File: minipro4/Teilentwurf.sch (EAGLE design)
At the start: 90 parts, among them IC1 MEGA8-P, IC2 FT232RL_ADAPTER, IC3 78L08Z, IC4 4051N, IC5 TL082P, IC6 4051N, IC7 TL082P, J1 HOHLSTECKER, Q2 BS170, Q3 BS170, Q4 BS170, Q6 IRF4905, X1 , X2 CON_COAX

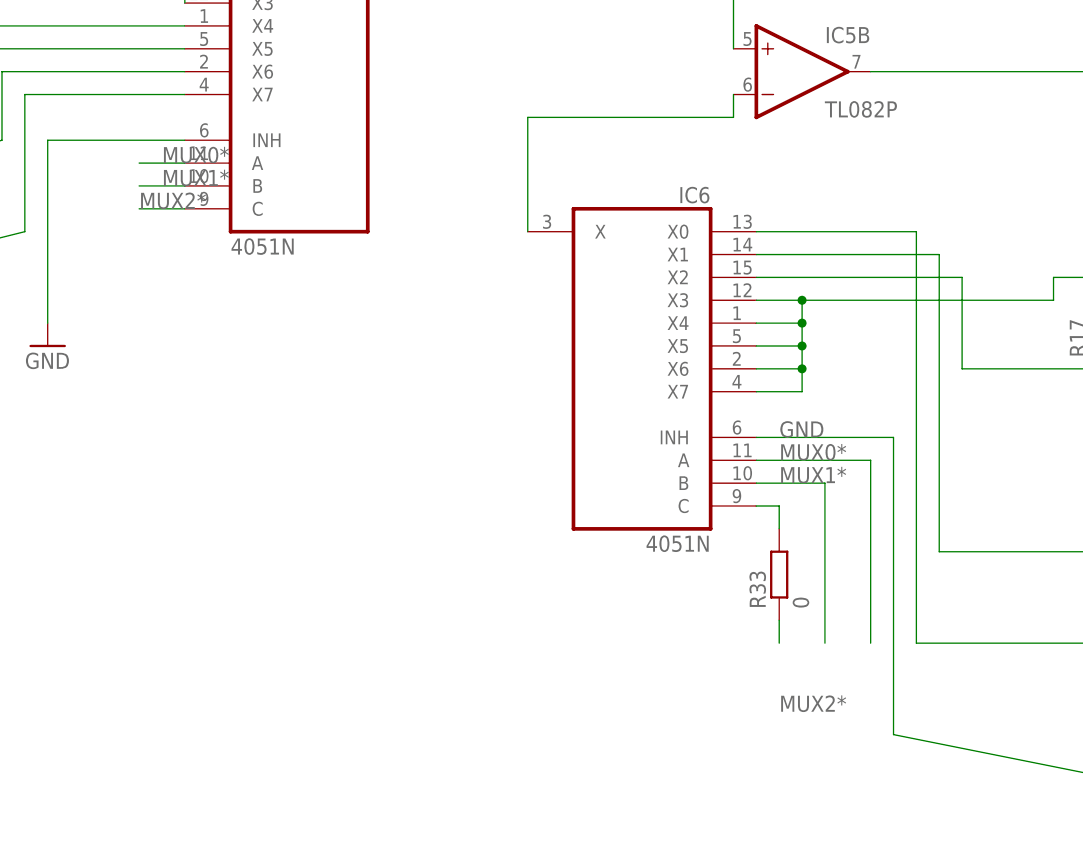
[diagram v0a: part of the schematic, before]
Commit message: Layout Iteration
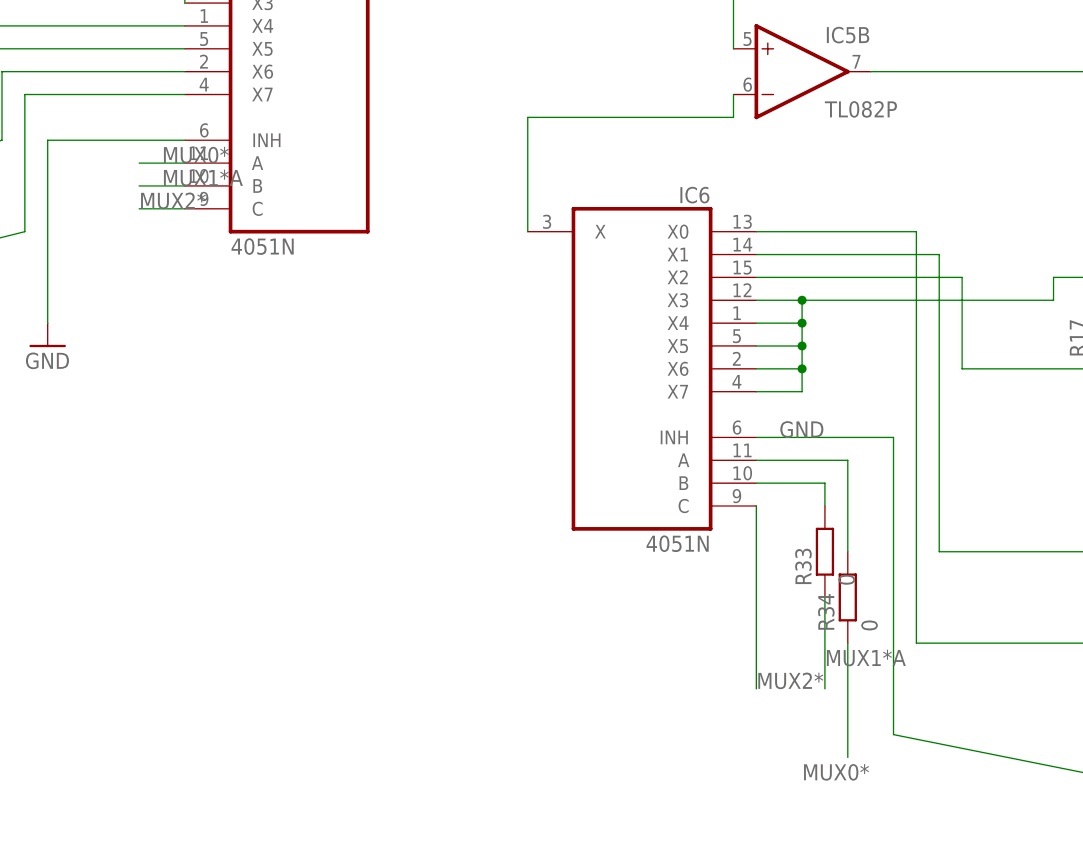
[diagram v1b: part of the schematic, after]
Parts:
- added R34: 0, 03_device-library:R-EU_0207/10
- R25: device 03_device-library:R-EU_0207/10 -> resistor:R-EU_0207/7
- R28: device 03_device-library:R-EU_0207/15 -> 03_device-library:R-EU_0207/10
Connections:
- removed net N$42: IC6A.C, R33.2
- new net MUX1*A: IC4A.B, R33.1
- new net N$45: IC6A.A, R34.2
- net MUX0*: now also R34.1; no longer IC6A.A
- net MUX1*: now also R33.2; no longer IC4A.B
- net MUX2*: now also IC6A.C; no longer R33.1
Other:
- moved on the sheet: R33
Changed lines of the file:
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@@
 <part name="GND16" library="03_device-library" deviceset="GND" device=""/>
 <part name="IC7" library="03_device-library" deviceset="TL082" device="P"/>
-<part name="R25" library="03_device-library" deviceset="R-EU_" device="0207/10" value="100k"/>
+<part name="R25" library="resistor" deviceset="R-EU_" device="0207/7" value="100k"/>
 <part name="P+4" library="03_device-library" deviceset="V+" device=""/>
 <part name="P-2" library="03_device-library" deviceset="V-" device=""/>
 <part name="R26" library="03_device-library" deviceset="POT" device="" value="100k"/>
 <part name="R27" library="03_device-library" deviceset="R-EU_" device="0207/10" value="22k"/>
-<part name="R28" library="03_device-library" deviceset="R-EU_" device="0207/15" value="8k2"/>
+<part name="R28" library="03_device-library" deviceset="R-EU_" device="0207/10" value="8k2"/>
 <part name="R32" library="03_device-library" deviceset="R-EU_" device="0207/15" value="220"/>
 <part name="C17" library="03_device-library" deviceset="C-EU" device="025-030X050" value="1nF"/>
@@
 <part name="GND21" library="03_device-library" deviceset="GND" device=""/>
 <part name="R33" library="03_device-library" deviceset="R-EU_" device="0207/10" value="0"/>
+<part name="R34" library="03_device-library" deviceset="R-EU_" device="0207/10" value="0"/>
 </parts>
 <sheets>
@@
 <instance part="GND20" gate="1" x="365.76" y="60.96"/>
 <instance part="GND21" gate="1" x="403.86" y="58.42"/>
-<instance part="R33" gate="G$1" x="160.02" y="-86.36" rot="R90"/>
+<instance part="R33" gate="G$1" x="165.1" y="-83.82" rot="R90"/>
+<instance part="R34" gate="G$1" x="167.64" y="-88.9" rot="R90"/>
 </instances>
 <busses>
@@
 </segment>
 <segment>
-<pinref part="IC6" gate="A" pin="A"/>
-<wire x1="157.48" y1="-73.66" x2="170.18" y2="-73.66" width="0.1524" layer="91"/>
-<wire x1="170.18" y1="-73.66" x2="170.18" y2="-93.98" width="0.1524" layer="91"/>
-<label x="160.02" y="-73.66" size="1.778" layer="95"/>
+<pinref part="R34" gate="G$1" pin="1"/>
+<wire x1="167.64" y1="-93.98" x2="167.64" y2="-106.68" width="0.1524" layer="91"/>
+<label x="162.56" y="-109.22" size="1.778" layer="95"/>
 </segment>
 </net>
@@
 </segment>
 <segment>
-<pinref part="R33" gate="G$1" pin="1"/>
-<wire x1="160.02" y1="-91.44" x2="160.02" y2="-93.98" width="0.1524" layer="91"/>
-<label x="160.02" y="-101.6" size="1.778" layer="95"/>
+<pinref part="IC6" gate="A" pin="C"/>
+<wire x1="157.48" y1="-78.74" x2="157.48" y2="-99.06" width="0.1524" layer="91"/>
+<label x="157.48" y="-99.06" size="1.778" layer="95"/>
 </segment>
 </net>
@@
 </segment>
 <segment>
-<pinref part="IC4" gate="A" pin="B"/>
-<wire x1="93.98" y1="-43.18" x2="88.9" y2="-43.18" width="0.1524" layer="91"/>
-<label x="91.44" y="-43.18" size="1.778" layer="95"/>
-</segment>
-<segment>
 <pinref part="IC6" gate="A" pin="B"/>
+<pinref part="R33" gate="G$1" pin="2"/>
 <wire x1="157.48" y1="-76.2" x2="165.1" y2="-76.2" width="0.1524" layer="91"/>
-<wire x1="165.1" y1="-76.2" x2="165.1" y2="-93.98" width="0.1524" layer="91"/>
-<label x="160.02" y="-76.2" size="1.778" layer="95"/>
+<wire x1="165.1" y1="-76.2" x2="165.1" y2="-78.74" width="0.1524" layer="91"/>
 </segment>
 </net>
@@
 </segment>
 </net>
-<net name="N$42" class="0">
-<segment>
-<pinref part="IC6" gate="A" pin="C"/>
-<wire x1="157.48" y1="-78.74" x2="160.02" y2="-78.74" width="0.1524" layer="91"/>
-<pinref part="R33" gate="G$1" pin="2"/>
-<wire x1="160.02" y1="-78.74" x2="160.02" y2="-81.28" width="0.1524" layer="91"/>
-</segment>
-</net>
+<net name="N$45" class="0">
+<segment>
+<pinref part="IC6" gate="A" pin="A"/>
+<pinref part="R34" gate="G$1" pin="2"/>
+<wire x1="157.48" y1="-73.66" x2="167.64" y2="-73.66" width="0.1524" layer="91"/>
+<wire x1="167.64" y1="-73.66" x2="167.64" y2="-83.82" width="0.1524" layer="91"/>
+</segment>
+</net>
+<net name="MUX1*A" class="0">
+<segment>
+<pinref part="R33" gate="G$1" pin="1"/>
+<wire x1="165.1" y1="-88.9" x2="165.1" y2="-99.06" width="0.1524" layer="91"/>
+<label x="165.1" y="-96.52" size="1.778" layer="95"/>
+</segment>
+<segment>
+<pinref part="IC4" gate="A" pin="B"/>
+<wire x1="93.98" y1="-43.18" x2="88.9" y2="-43.18" width="0.1524" layer="91"/>
+<label x="91.44" y="-43.18" size="1.778" layer="95"/>
+</segment>
+</net>
